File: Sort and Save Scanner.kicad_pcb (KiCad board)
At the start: 4 copper layers, 132.1 x 86.4 mm, 60 parts, among them J201 B4B-PH-K-S_LF__SN_, J301 FTSH-105-01-F-DV-K, J302 FTSH-105-01-F-DV-K, J401 67996-412HLF, U201 LM78L12_SO8, U202 LT1763CS8-5, U203 LT1763CS8-3.3, U301 STM32F051R8Tx, U401 OPA2376AIDR-8, U402 REF5025AD, Y301 8MHz

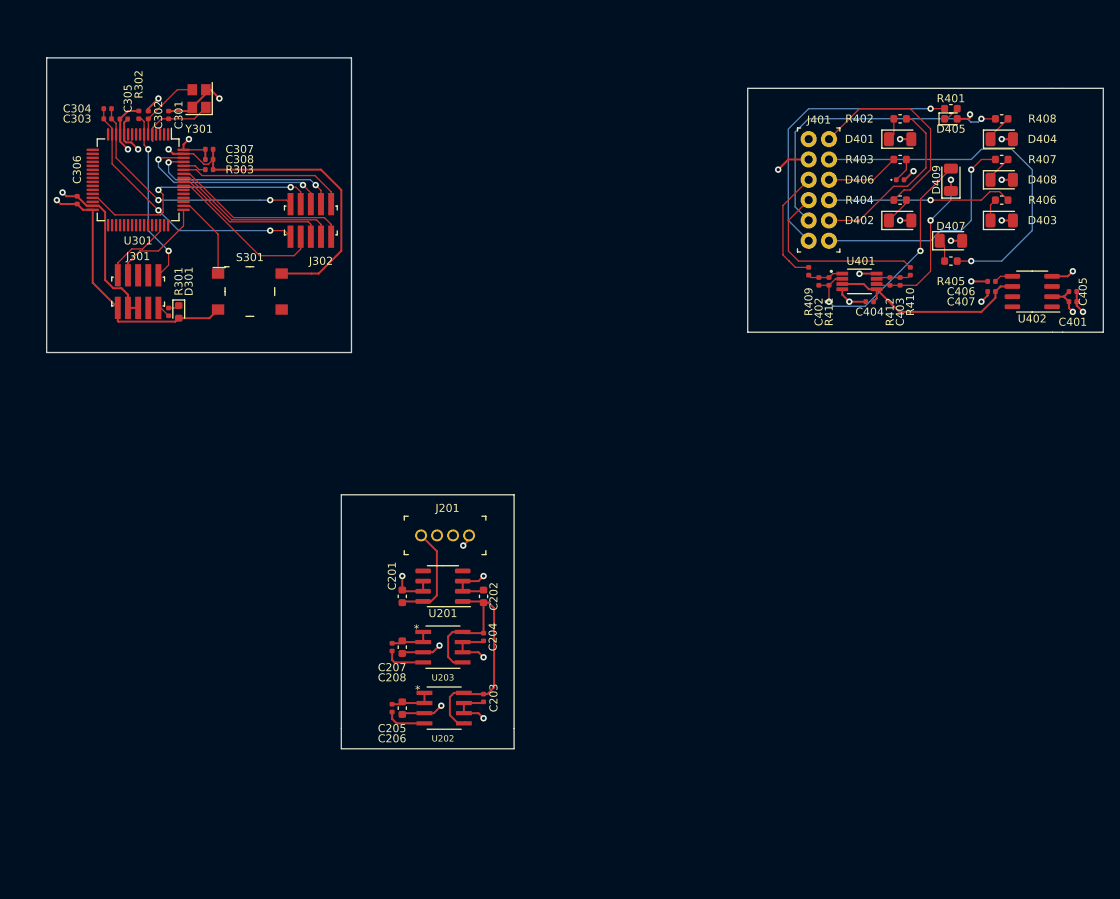
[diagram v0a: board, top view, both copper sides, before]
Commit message: v1.0.0
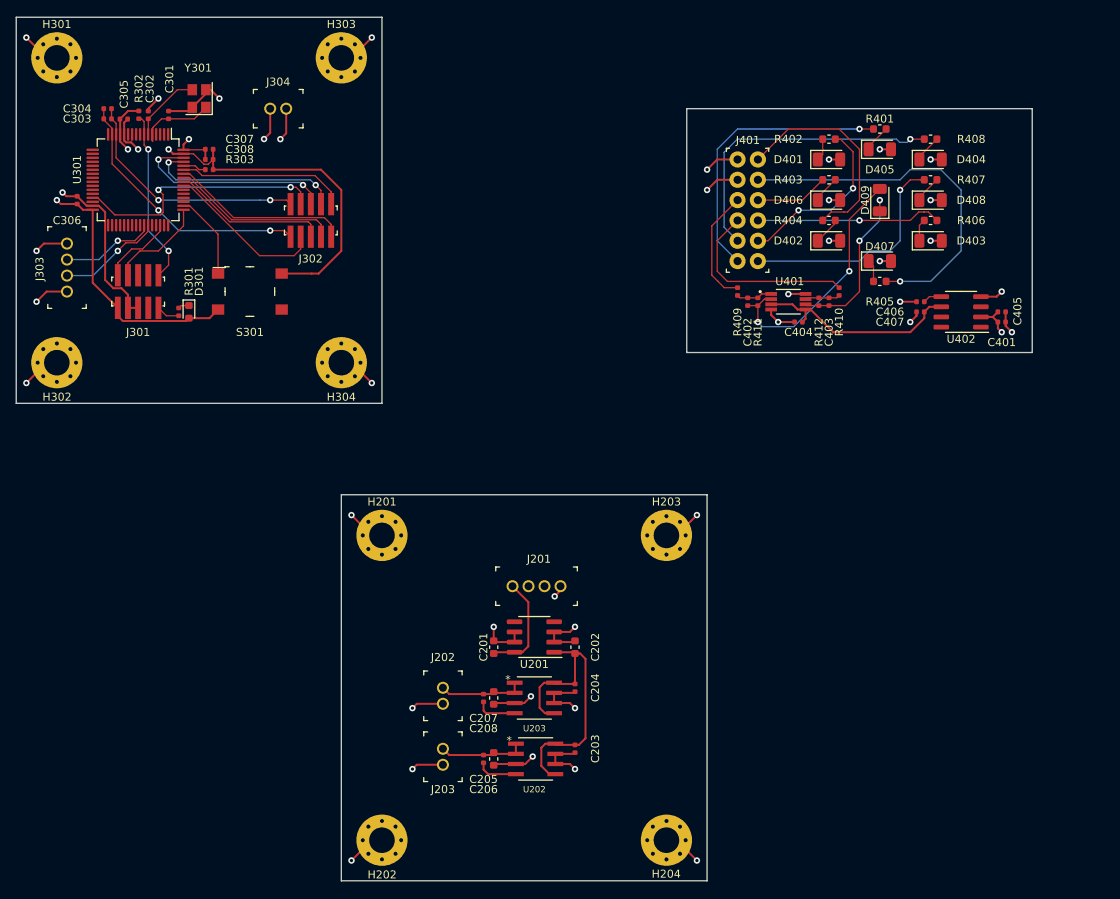
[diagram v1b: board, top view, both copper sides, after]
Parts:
- added H201: MountingHole_Pad, MountingHole:MountingHole_3.2mm_M3_Pad_Via, F.Cu at (119.4, 128.3)
- added H202: MountingHole_Pad, MountingHole:MountingHole_3.2mm_M3_Pad_Via, F.Cu at (119.4, 166.4)
- added H203: MountingHole_Pad, MountingHole:MountingHole_3.2mm_M3_Pad_Via, F.Cu at (154.9, 128.3)
- added H204: MountingHole_Pad, MountingHole:MountingHole_3.2mm_M3_Pad_Via, F.Cu at (154.9, 166.4)
- added H301: MountingHole_Pad, MountingHole:MountingHole_3.2mm_M3_Pad_Via, F.Cu at (78.7, 68.6)
- added H302: MountingHole_Pad, MountingHole:MountingHole_3.2mm_M3_Pad_Via, F.Cu at (78.7, 106.7)
- added H303: MountingHole_Pad, MountingHole:MountingHole_3.2mm_M3_Pad_Via, F.Cu at (114.3, 68.6)
- added H304: MountingHole_Pad, MountingHole:MountingHole_3.2mm_M3_Pad_Via, F.Cu at (114.3, 106.7)
- added J202: B2B-PH-K-S_LF__SN_, digikey-footprints:PinHeader_1x2_P2mm_Drill1mm, F.Cu at (127.0, 147.3)
- added J203: B2B-PH-K-S_LF__SN_, digikey-footprints:PinHeader_1x2_P2mm_Drill1mm, F.Cu at (127.0, 154.9)
- added J303: B4B-PH-K-S_LF__SN_, digikey-footprints:PinHeader_1x4_P2mm_Drill1mm, F.Cu at (80.0, 97.8)
- added J304: B2B-PH-K-S_LF__SN_, digikey-footprints:PinHeader_1x2_P2mm_Drill1mm, F.Cu at (105.4, 74.9)
- D405: footprint LED_SMD:LED_0603_1608Metric -> LED_SMD:LED_1206_3216Metric
- D406: value 950nm -> 940nm; footprint LED_SMD:LED_0402_1005Metric -> LED_SMD:LED_1206_3216Metric
- R402: value 39 -> 66
- moved C201 13.1 mm to (133.3, 142.2)
- moved C205 13.1 mm to (132.1, 156.2)
- moved C207 13.1 mm to (132.1, 148.6)
- moved U201 13.1 mm to (138.4, 141.0)
- moved U203 13.1 mm to (138.4, 148.6)
- moved C206 13.1 mm to (133.3, 156.2)
- moved C208 13.1 mm to (133.3, 148.6)
- moved J201 13.1 mm to (135.7, 134.6)
- moved U202 13.1 mm to (138.6, 156.2)
- moved C202 13.1 mm to (143.5, 142.2)
- moved C203 13.1 mm to (143.5, 154.9)
- moved C204 13.1 mm to (143.5, 147.3)
- moved D405 9.67 mm to (181.6, 80.0)
- moved C402 9.25 mm to (165.1, 99.1)
- moved C403 9.25 mm to (175.3, 99.1)
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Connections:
- J401 pad 1: Net-(J401-Pad1) -> GND
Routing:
- net GND: track 142.7 -> 201.6 mm, vias 25 -> 38
- net +3V3: track 63.3 -> 76.6 mm, vias 3 -> 5
- net /ARM Board/UART_TX: track 0.00 -> 13.2 mm, vias 0 -> 1
- net /ARM Board/UART_RX: track 0.00 -> 11.9 mm, vias 0 -> 1
- net +5V: track 16.8 -> 22.2 mm
- net Net-(J301-Pad9): track 1.68 -> 3.23 mm
- net Net-(D405-Pad1): track 2.10 -> 3.45 mm
- net /Sensor/LED_PWR_IN5: track 27.0 -> 27.8 mm
- net /Sensor/LED_PWR_IN7: track 22.4 -> 22.0 mm, vias 0 -> 2
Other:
- board size 132.1 x 86.4 mm -> 127 x 107.9 mm
